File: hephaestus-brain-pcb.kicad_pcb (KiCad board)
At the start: 2 copper layers, 19.1 x 64.8 mm, 11 parts, among them J1 Barrel_Jack, J2 ItsyBitsy, J3 ItsyBitsy, J4 Conn_01x03_Male, J5 Conn_01x03_Male, J6 Conn_01x03_Male, J7 Conn_01x03_Male, J8 Conn_01x02_Female, U1 74126

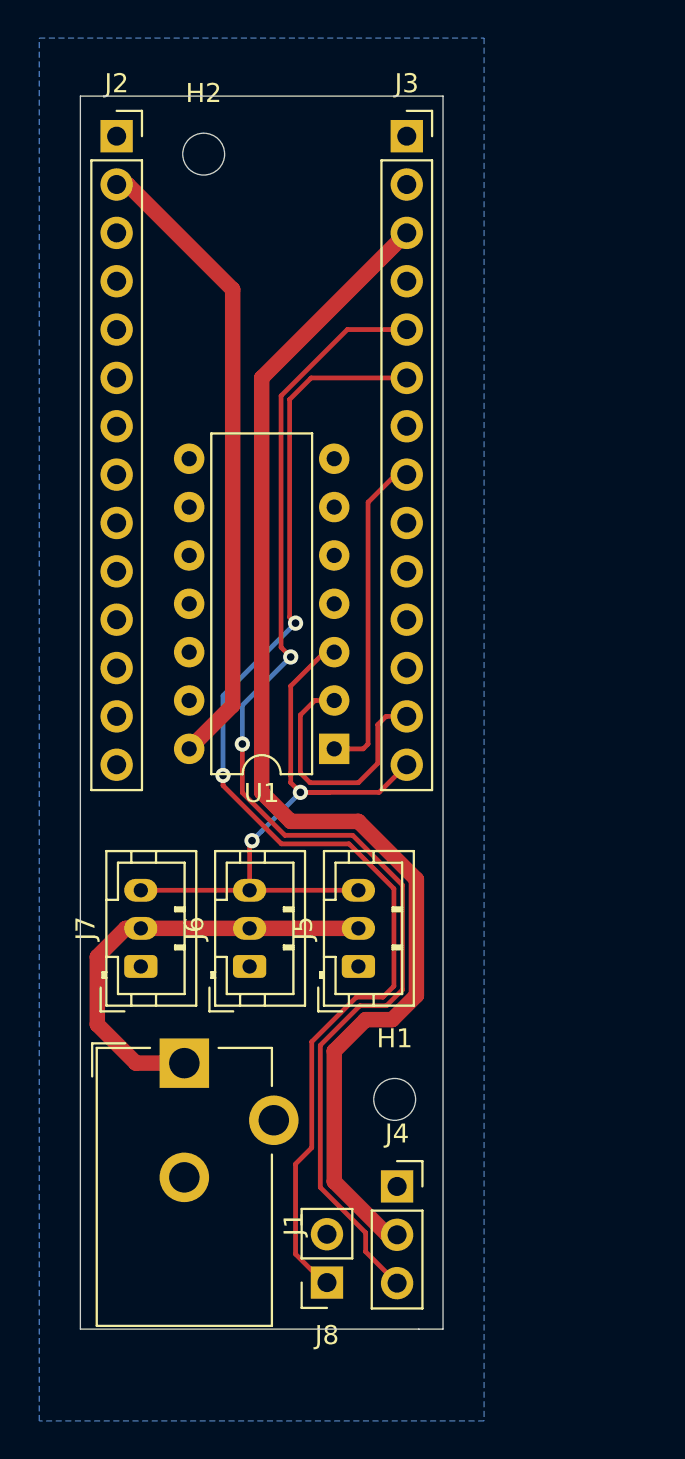
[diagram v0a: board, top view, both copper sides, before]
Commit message: Added switch, button.
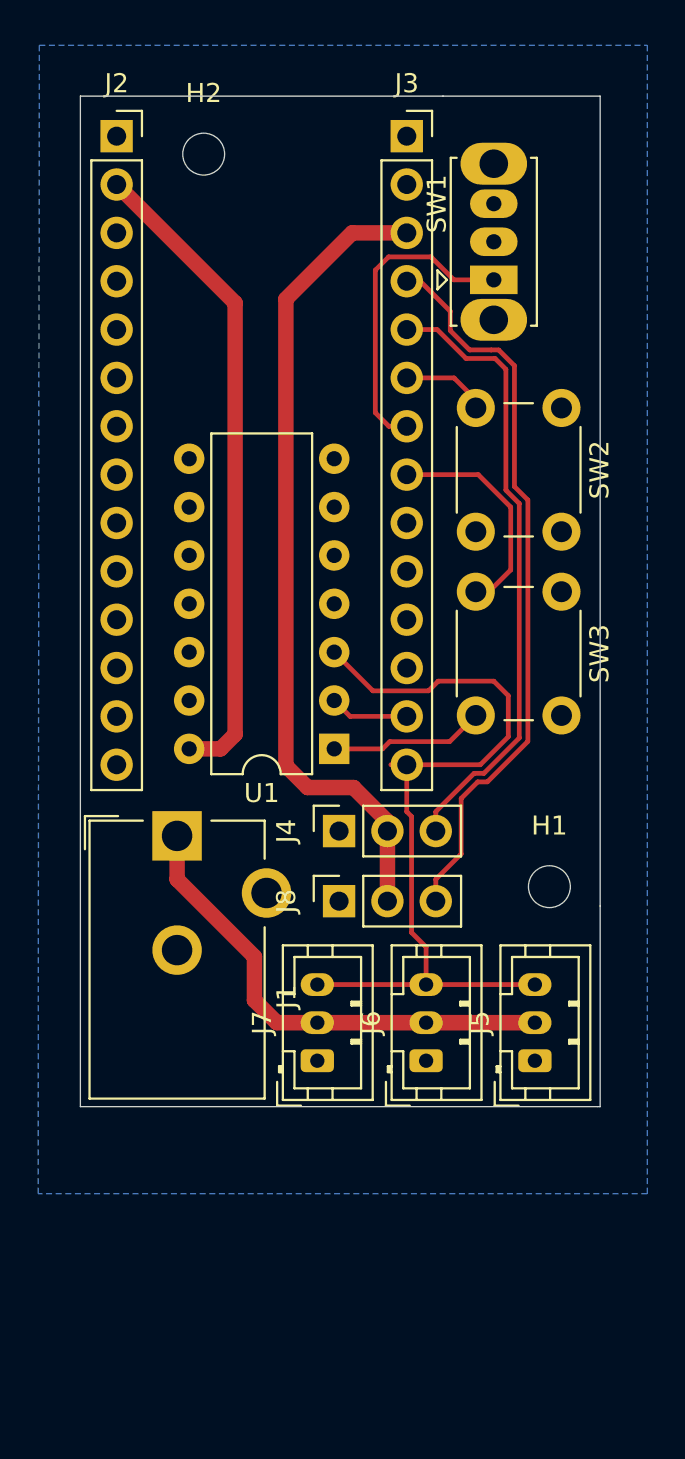
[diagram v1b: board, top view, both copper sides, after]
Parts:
- added SW1: SW_SPDT, Button_Switch_THT:SW_Slide_1P2T_CK_OS102011MS2Q, F.Cu at (184.9, 70.6)
- added SW2: SW_SPST, Button_Switch_THT:SW_PUSH_6mm, F.Cu at (188.5, 77.3)
- added SW3: SW_SPST, Button_Switch_THT:SW_PUSH_6mm, F.Cu at (188.5, 87.0)
- J8: value Conn_01x02_Female -> Conn_01x03_Male; footprint Connector_PinSocket_2.54mm:PinSocket_1x02_P2.54mm_Vertical -> Connector_PinSocket_2.54mm:PinSocket_1x03_P2.54mm_Vertical
- moved J8 20.0 mm to (176.8, 103.3), turned to 90 degrees
- moved J4 18.9 mm to (176.8, 99.6), turned to 90 degrees
- moved H1 13.8 mm to (187.8, 102.5)
- moved J1 11.9 mm to (168.3, 99.8)
- moved J5 10.5 mm to (187.1, 111.6)
- moved J6 10.5 mm to (181.4, 111.6)
- moved J7 10.5 mm to (175.6, 111.6)
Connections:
- J8 pad 1: 11 -> GND
- J8 pad 2: GND -> USB
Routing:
- net 11: track 64.3 -> 4.54 mm, vias 2 -> 0
- net 13: track 0.00 -> 38.8 mm
- net 12: track 65.8 -> 32.7 mm, vias 2 -> 0
- net USB: track 65.5 -> 43.0 mm
- net 10: track 0.00 -> 16.4 mm
- net TX: track 13.6 -> 4.16 mm
- net RX: track 33.8 -> 42.8 mm, vias 2 -> 0
- net 9: track 17.2 -> 19.9 mm
- net VPOW: track 23.6 -> 25.5 mm
- net 3v: track 33.5 -> 34.2 mm
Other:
- board size 19.1 x 64.8 mm -> 27.3 x 53.1 mm
